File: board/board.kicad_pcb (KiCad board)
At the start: 2 copper layers, 71.4 x 59 mm, 81 parts, among them J1 Molex Picoblade, J2 Conn_ARM_JTAG_SWD_10, J3 USB_B_Micro, J4 Conn_01x04_Male, J5 Screw_Terminal_01x02, Q2 Q_NMOS_GDS, Q3 Q_NMOS_GDS, Q4 Q_NMOS_GDS, Q5 Find one, U1 STM32F405RGTx, U2 TPS542941, U3 ELVH-100A-HANH-C-N2A5, U4 UCC2751x, U5 MX25R3235FM2xx1, U6 USBLC6-2SC6, Y1 16MHz

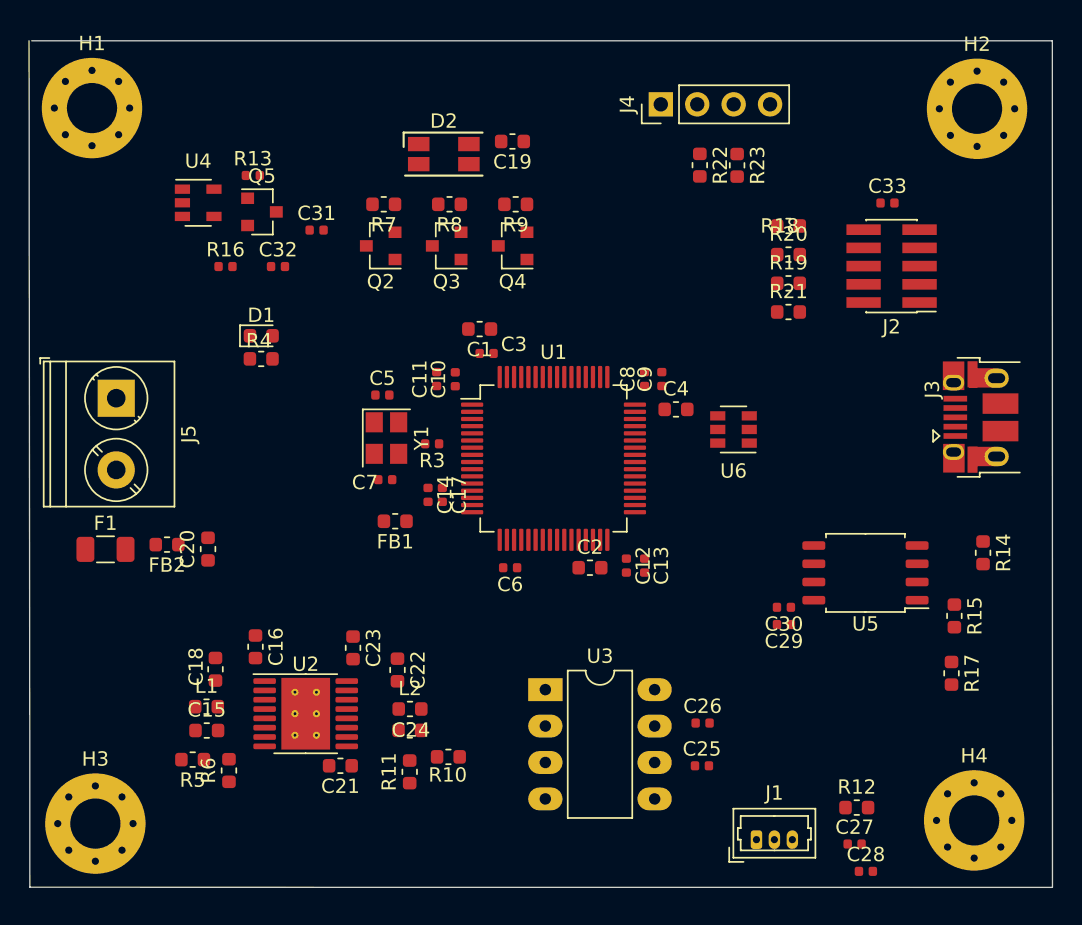
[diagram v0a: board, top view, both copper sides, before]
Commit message: Update
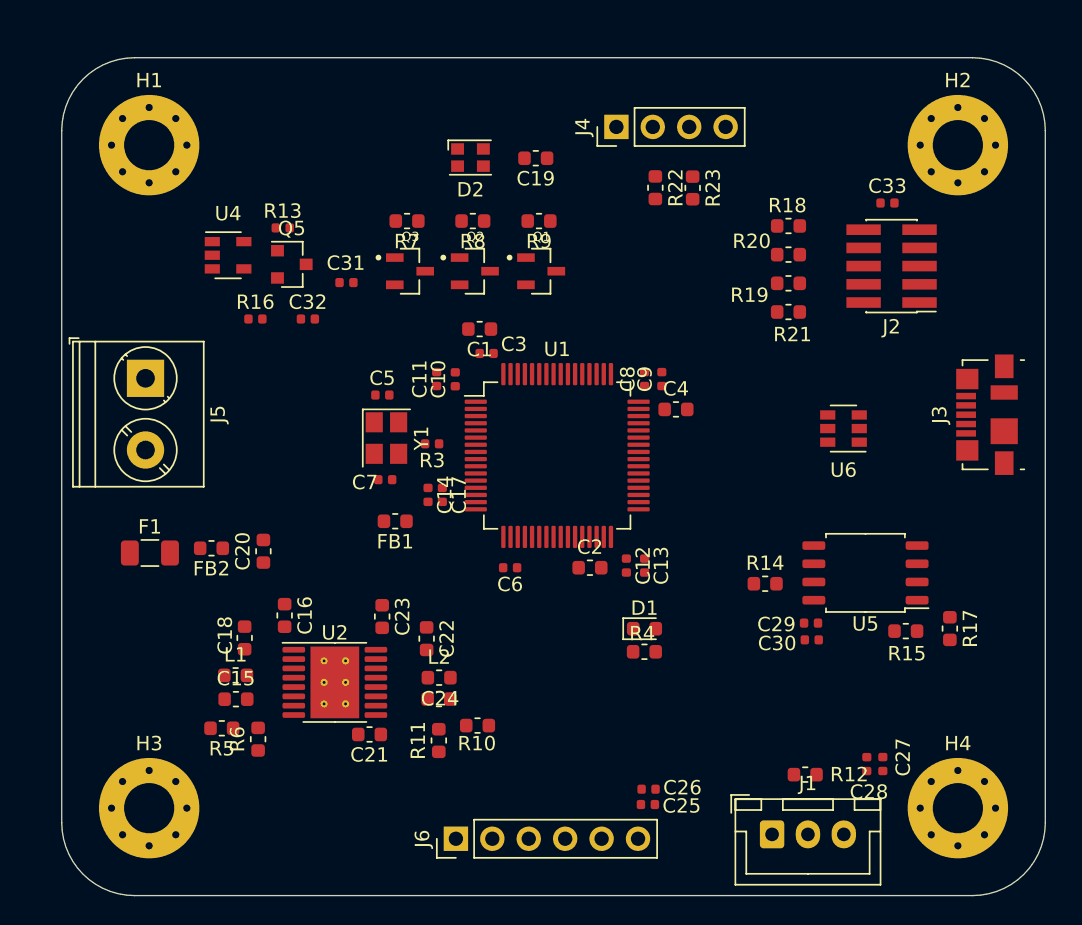
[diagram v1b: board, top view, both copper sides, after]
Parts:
- removed Q4: Q_NMOS_GDS, Package_TO_SOT_SMD:SOT-23
- removed U3: ELVH-100A-HANH-C-N2A5, Package_DIP:DIP-8_W7.62mm_LongPads
- added J6: Conn_01x06_Male, Connector_PinHeader_2.54mm:PinHeader_1x06_P2.54mm_Vertical, F.Cu at (88.4, 135.7)
- added Q1: FDV305N, SOT95P240X111-3N, F.Cu at (94.4, 96.2)
- D2: value LED_RGB -> ASMB-KTF0-0A306; footprint LED_SMD:LED_RGB_1210 -> LED_SMD:LED_ASMB-KTF0-0A306
- J1: footprint Connector_Molex:Molex_PicoBlade_53047-0310_1x03_P1.25mm_Vertical -> Connector_JST:JST_XH_B3B-XH-A_1x03_P2.50mm_Vertical
- J3: footprint Connector_USB:USB_Micro-B_Amphenol_10103594-0001LF_Horizontal -> Connector_USB:USB_Micro-B_Molex_47346-0001
- Q2, Q3: value Q_NMOS_GDS -> FDV305N; footprint Package_TO_SOT_SMD:SOT-23 -> SOT95P240X111-3N
- moved D1 33.6 mm to (101.6, 121.1)
- moved R4 33.6 mm to (101.6, 122.7)
- moved R14 15.3 mm to (110.0, 118.0), turned to 0 degrees
- moved U6 7.67 mm to (115.5, 107.1)
- moved C28 7.48 mm to (117.1, 130.5), turned to 90 degrees
- moved Q2 6.80 mm to (89.8, 96.2), turned to 0 degrees
- moved C26 5.96 mm to (101.9, 132.3)
- moved C27 5.91 mm to (118.2, 130.5), turned to 270 degrees
- moved H1 4.75 mm to (67.1, 87.4)
- moved C25 4.64 mm to (101.8, 133.3)
- moved R12 4.27 mm to (112.8, 131.3)
- moved R13 4.21 mm to (76.4, 93.1)
- moved R16 4.21 mm to (74.5, 99.5)
- moved U4 4.21 mm to (72.6, 95.1)
- moved C31 4.21 mm to (80.8, 97.0)
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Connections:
- D2 pad 1: Net-(D2-Pad1) -> +3V3
- D2 pad 4: +3V3 -> Net-(D2-Pad4)
- F1 pad 1: +UCC_VDD -> Net-(F1-Pad1)
- F1 pad 2: Net-(F1-Pad2) -> +UCC_VDD
- Q2 pad 1: TIM4_CH1 -> TIM4_CH2
- Q2 pad 2: Net-(Q2-Pad2) -> PGND1
- Q2 pad 3: PGND1 -> Net-(Q2-Pad3)
- Q3 pad 1: TIM4_CH2 -> TIM4_CH3
- Q3 pad 2: Net-(Q3-Pad2) -> PGND1
- Q3 pad 3: PGND1 -> Net-(Q3-Pad3)
- R7 pad 1: Net-(Q2-Pad2) -> Net-(Q1-Pad3)
- R7 pad 2: Net-(D2-Pad1) -> Net-(D2-Pad2)
- R8 pad 1: Net-(Q3-Pad2) -> Net-(Q2-Pad3)
- R8 pad 2: Net-(D2-Pad2) -> Net-(D2-Pad4)
- R9 pad 1: Net-(Q4-Pad2) -> Net-(Q3-Pad3)
- U1 pad 51: Net-(R1-Pad2) -> USART3_TX
- U1 pad 52: Net-(R2-Pad2) -> USART3_RX
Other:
- board size 71.4 x 59 mm -> 68.6 x 58.4 mm
- copper layers 2 -> 4
